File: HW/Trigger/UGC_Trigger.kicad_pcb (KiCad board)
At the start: 2 copper layers, 9.3 x 19.1 mm, 3 parts, among them J1 Conn_01x01_Pin, J2 Conn_01x01_Pin, SW1 SW_Push

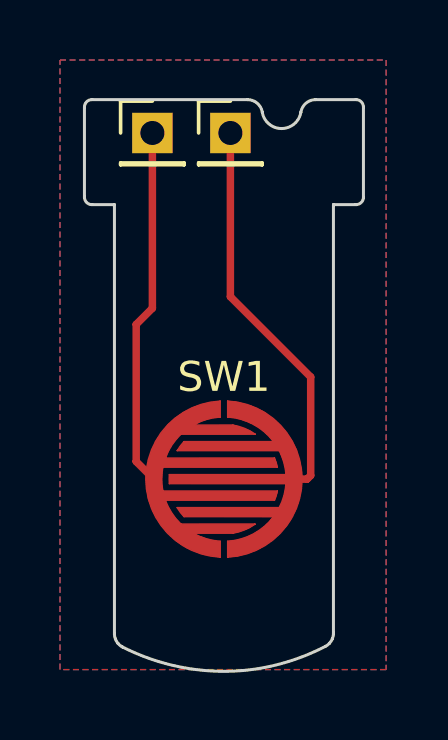
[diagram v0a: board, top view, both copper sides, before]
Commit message: Production files
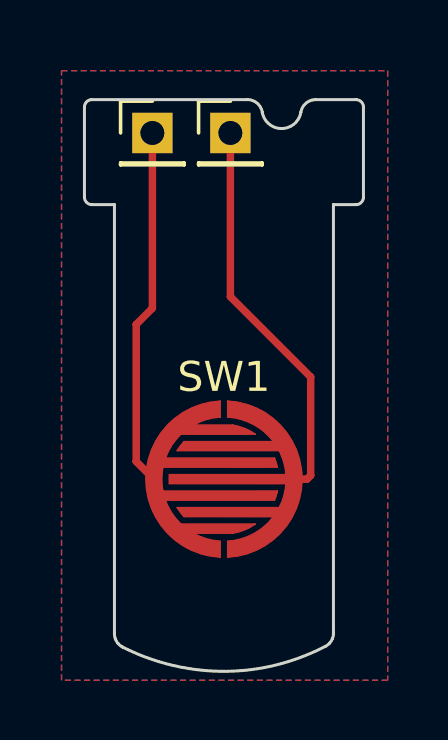
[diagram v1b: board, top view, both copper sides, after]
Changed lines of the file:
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@@
     (fp_arc (start -1.844542 0.949938) (mid -1.997407 0.561307) (end -2.069357 0.149938)
       (stroke (width 0.05) (type solid)) (layer "F.Cu"))
-    (fp_arc (start -1.780411 -0.400062) (mid -1.739286 -0.552119) (end -1.685201 -0.700062)
-      (stroke (width 0.05) (type solid)) (layer "F.Cu"))
-    (fp_arc (start -1.685201 0.699938) (mid -1.739284 0.551994) (end -1.780411 0.399938)
+    (fp_arc (start -1.780411 -0.400062) (mid -1.739284 -0.552118) (end -1.685201 -0.700062)
+      (stroke (width 0.05) (type solid)) (layer "F.Cu"))
+    (fp_arc (start -1.685201 0.699938) (mid -1.739285 0.551994) (end -1.780411 0.399938)
       (stroke (width 0.05) (type solid)) (layer "F.Cu"))
     (fp_arc (start -1.656024 -1.250062) (mid -0.980504 -1.828673) (end -0.124786 -2.071294)
@@
     (fp_arc (start 1.433958 -1.500061) (mid 1.740364 -1.130327) (end 1.953577 -0.700062)
       (stroke (width 0.05) (type solid)) (layer "F.Cu"))
-    (fp_arc (start 1.558458 0.949938) (mid 1.451963 1.105859) (end 1.329923 1.249938)
+    (fp_arc (start 1.558458 0.949938) (mid 1.451962 1.105858) (end 1.329923 1.249938)
       (stroke (width 0.05) (type solid)) (layer "F.Cu"))
     (fp_arc (start 1.819039 -0.150062) (mid 1.825214 -0.000062) (end 1.819039 0.149938)
       (stroke (width 0.05) (type solid)) (layer "F.Cu"))
-    (fp_arc (start 1.953576 0.699938) (mid 1.740365 1.130204) (end 1.433958 1.499937)
+    (fp_arc (start 1.953576 0.699938) (mid 1.740364 1.130203) (end 1.433958 1.499937)
       (stroke (width 0.05) (type solid)) (layer "F.Cu"))
     (fp_arc (start 2.036295 -0.400062) (mid 2.075214 -0.000062) (end 2.036295 0.399938)
@@
     (polygon
       (pts
-        (xy 273.4564 144.9832)
-        (xy 284.3276 144.9832)
-        (xy 284.3276 165.3032)
-        (xy 273.4564 165.3032)
+        (xy 273.5072 145.3388)
+        (xy 284.3784 145.3388)
+        (xy 284.3784 165.6588)
+        (xy 273.5072 165.6588)
       )
     )
